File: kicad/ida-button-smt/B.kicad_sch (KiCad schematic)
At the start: 19 parts, among them Q1 J113, SW3 ARCADE_BTN, U1 TL074, U2 40106

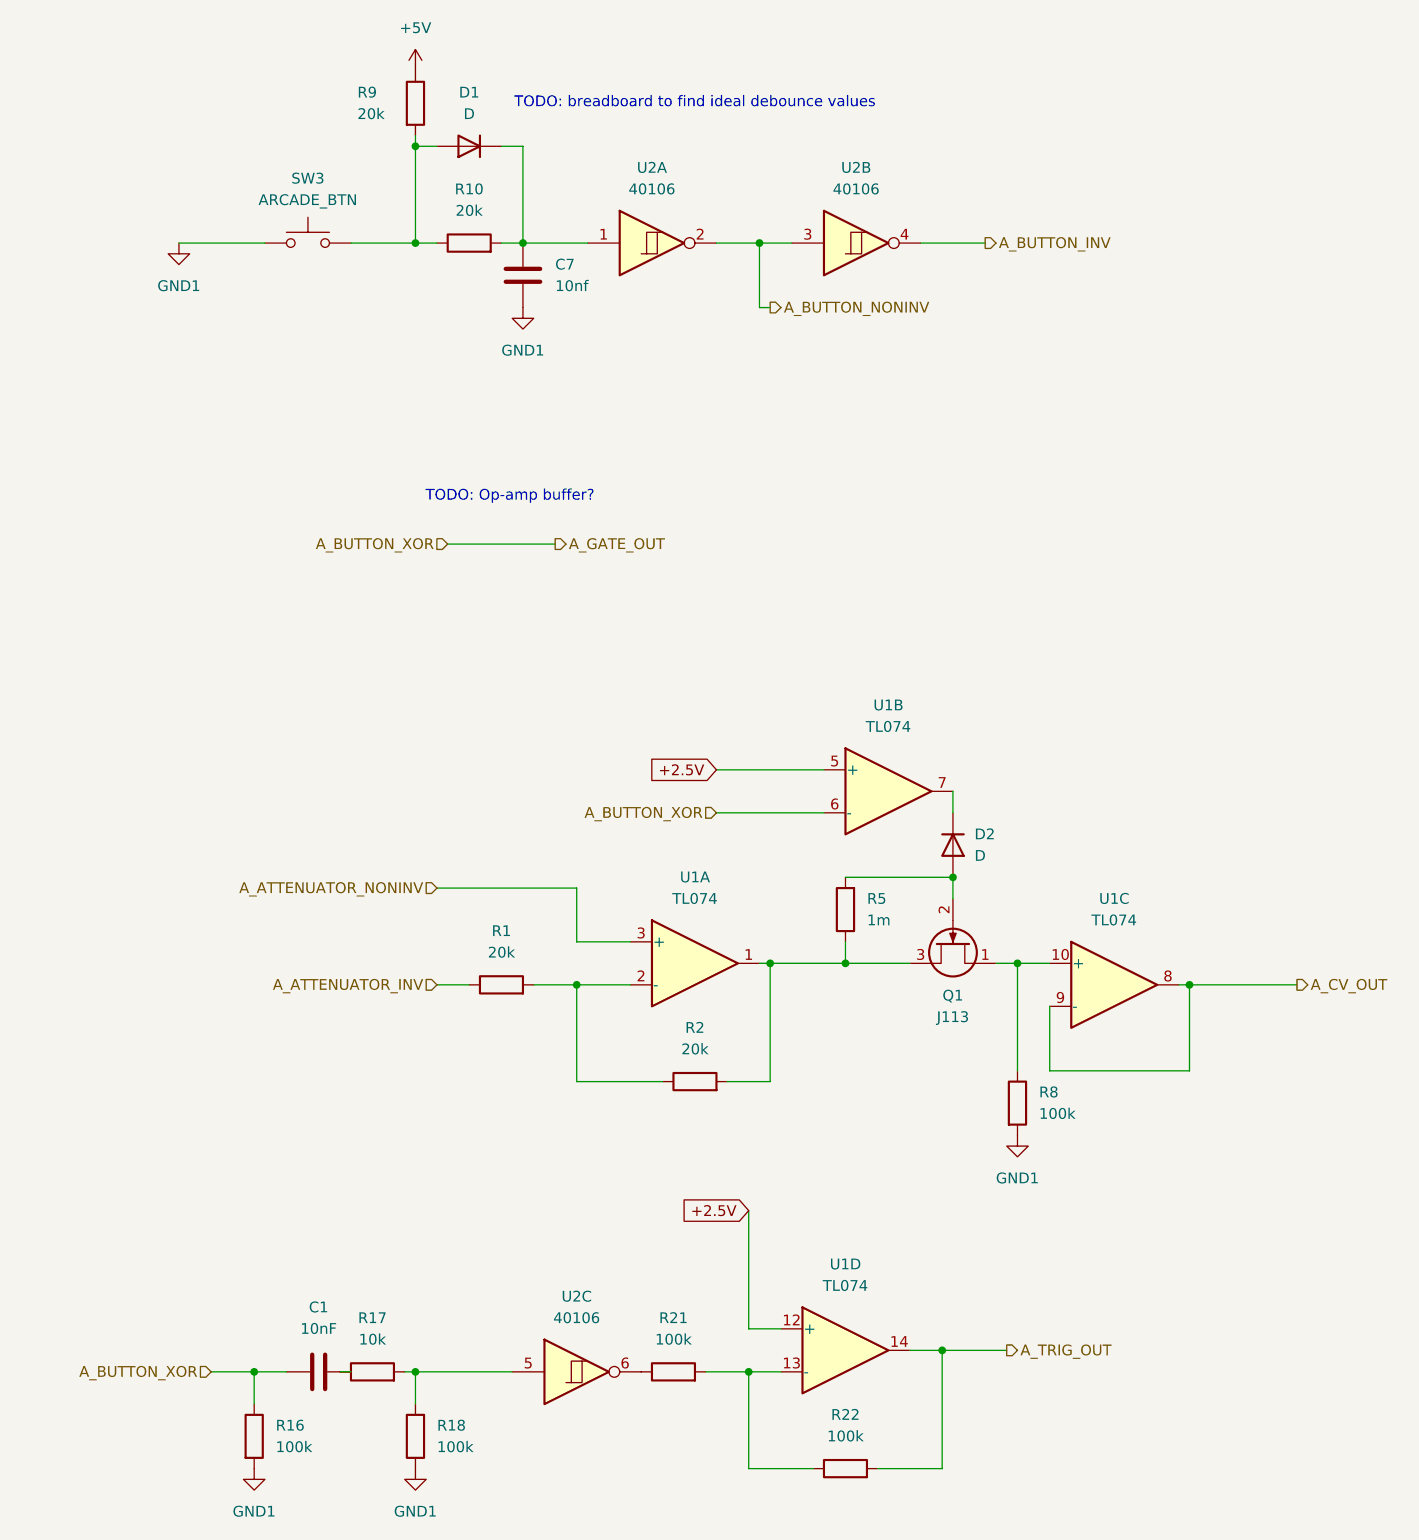
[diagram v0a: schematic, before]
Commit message: stylophone rev1
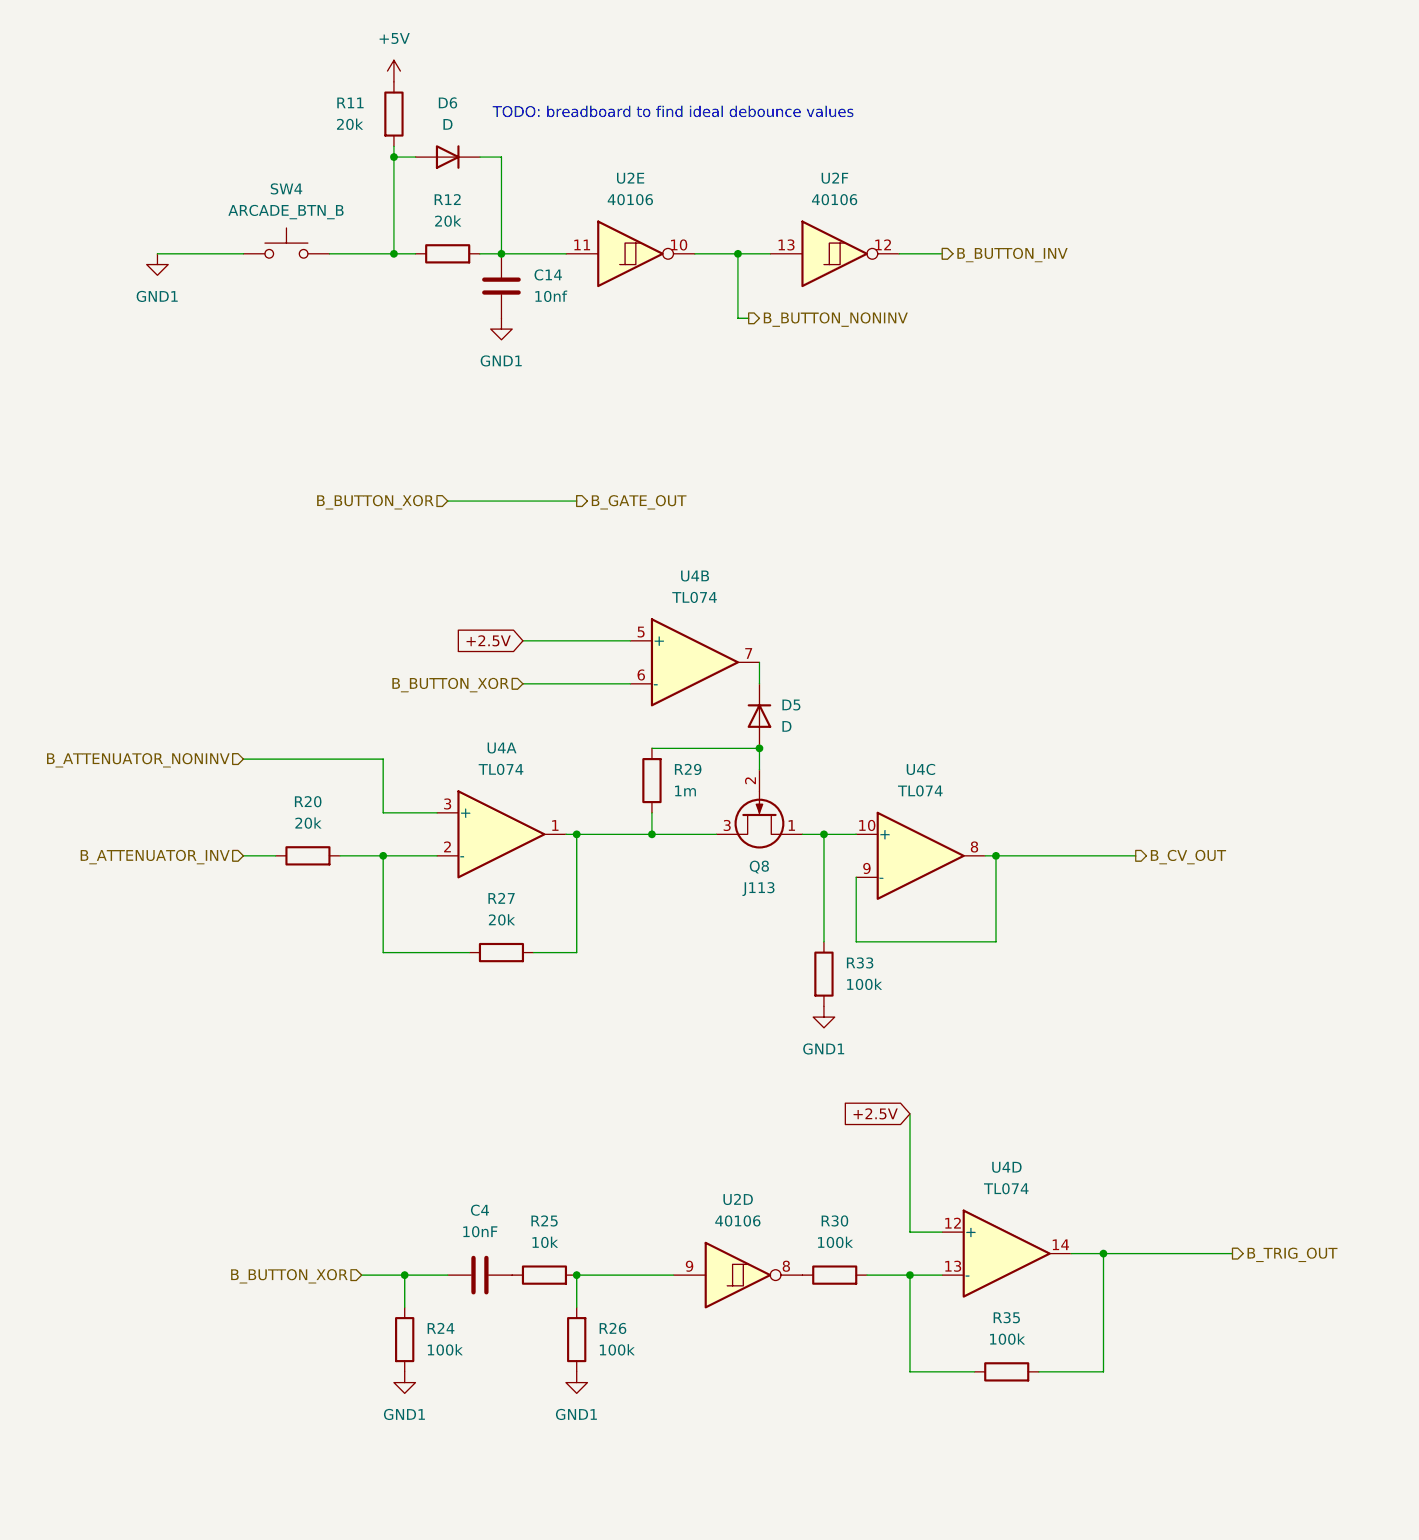
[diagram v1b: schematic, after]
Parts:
- removed C1: 10nF, PCM_4ms_Capacitor:C_Disc_P5.08mm, symbol Device:C
- removed C7: 10nf, PCM_4ms_Capacitor:C_Disc_P5.08mm, symbol Device:C
- removed D1, D2: D, PCM_4ms_Diode:D_DO-35_P7.62mm_Horizontal, symbol Device:D
- removed Q1: J113, Package_TO_SOT_THT:TO-92, symbol Transistor_FET:2N3819
- removed R1, R10, R2, R9: 20k, PCM_4ms_Resistor:R_Axial_DIN0207_L6.3mm_D2.5mm_P7.62mm_Horizontal, symbol Device:R
- removed R16, R18, R21, R22, R8: 100k, PCM_4ms_Resistor:R_Axial_DIN0207_L6.3mm_D2.5mm_P7.62mm_Horizontal, symbol Device:R
- removed R17: 10k, PCM_4ms_Resistor:R_Axial_DIN0207_L6.3mm_D2.5mm_P7.62mm_Horizontal, symbol Device:R
- removed R5: 1m, PCM_4ms_Resistor:R_Axial_DIN0207_L6.3mm_D2.5mm_P7.62mm_Horizontal, symbol Device:R
- removed SW3: ARCADE_BTN, Connector_JST:JST_XH_S2B-XH-A-1_1x02_P2.50mm_Horizontal, symbol Switch:SW_Push
- removed U1: TL074, Package_DIP:DIP-14_W7.62mm_Socket, symbol Amplifier_Operational:TL074
- removed U2: 40106, Package_DIP:DIP-14_W7.62mm_Socket, symbol 4xxx:40106
- added C14: 10nf, Capacitor_SMD:C_0603_1608Metric, symbol Device:C
- added C4: 10nF, Capacitor_SMD:C_0603_1608Metric, symbol Device:C
- added D5, D6: D, Diode_SMD:D_0603_1608Metric, symbol Device:D
- added Q8: J113, Package_TO_SOT_SMD:SOT-23_Handsoldering, symbol Transistor_FET:2N3819
- added R11, R12, R20, R27: 20k, Resistor_SMD:R_0603_1608Metric, symbol Device:R
- added R24, R26, R30, R33, R35: 100k, Resistor_SMD:R_0603_1608Metric, symbol Device:R
- added R25: 10k, Resistor_SMD:R_0603_1608Metric, symbol Device:R
- added R29: 1m, Resistor_SMD:R_0603_1608Metric, symbol Device:R
- added SW4: ARCADE_BTN_B, Connector_JST:JST_XH_S2B-XH-A-1_1x02_P2.50mm_Horizontal, symbol Switch:SW_Push
- added U2: 40106, Package_SO:TSSOP-14_4.4x5mm_P0.65mm, symbol 4xxx:40106
- added U4: TL074, Package_SO:SSOP-14_5.3x6.2mm_P0.65mm, symbol Amplifier_Operational:TL074
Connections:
- net +2.5V: now also U4.12 (+), U4.5 (+)
- net +5V: now also R11.1
- net GND1: now also C14.2, R24.2, R26.1, R33.2, SW4.1
- new net: C14.1, D6.1 (K), R12.2, U2.11
- new net: D5.1 (K), U4.7
- new net: D5.2 (A), Q8.2 (G), R29.2
- new net: R20.2, R27.1, U4.2 (-)
- new net: Q8.3 (S), R27.2, R29.1, U4.1
- new net: D6.2 (A), R11.2, R12.1, SW4.2
- new net: Q8.1 (D), R33.1, U4.10 (+)
- new net: R30.1, U2.8
- new net: R30.2, R35.1, U4.13 (-)
- new net: R25.2, R26.2, U2.9
- new net: C4.1, R25.1
- new net B_ATTENUATOR_INV: R20.1
- new net B_ATTENUATOR_NONINV: U4.3 (+)
- new net B_BUTTON_INV: U2.12
- new net B_BUTTON_NONINV: U2.10, U2.13
- new net B_BUTTON_XOR: C4.2, R24.1, U4.6 (-)
- new net B_CV_OUT: U4.8, U4.9 (-)
- new net B_TRIG_OUT: R35.2, U4.14
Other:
- note removed: "TODO: Op-amp buffer?"
